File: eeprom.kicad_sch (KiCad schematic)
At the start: 2 parts, among them U8 CAT25320VI-GT3

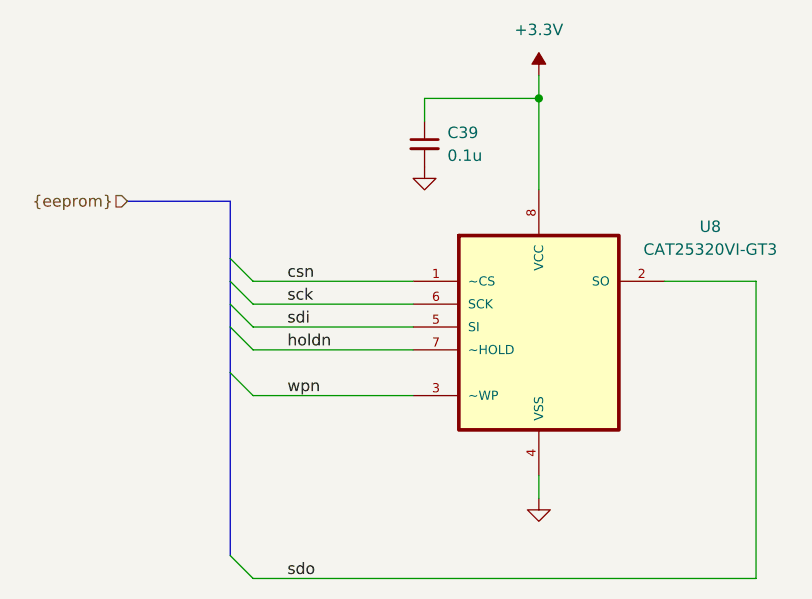
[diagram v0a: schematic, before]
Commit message: Finish BOM
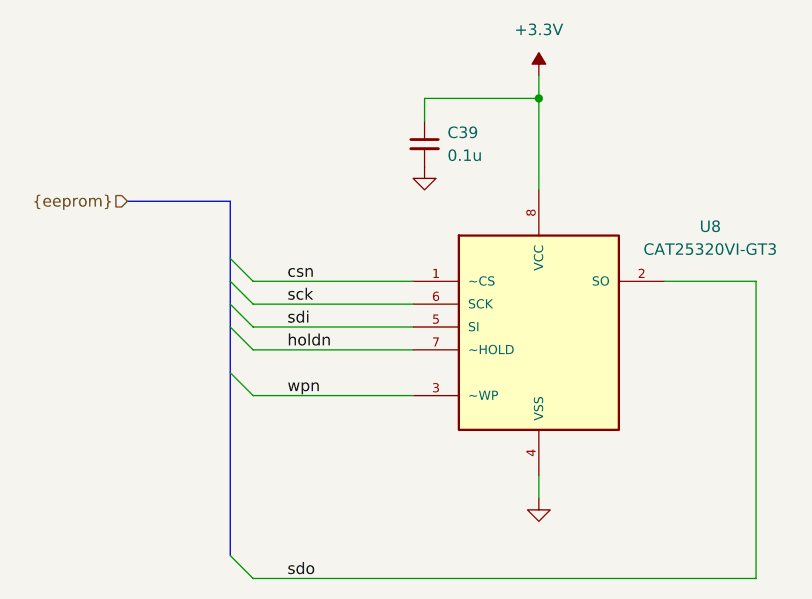
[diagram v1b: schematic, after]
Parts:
- C39: Cost (none) -> .08; MFG (none) -> Taiyo-Yuden; MFG_PN (none) -> TMF212B7104KGHT
- U8: Cost (none) -> 0.55; MFG ON Semiconductor -> ON Semi
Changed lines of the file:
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@@
 			)
 		)
-		(property "Description" "CAT25320VI-GT3 EEPROM Memory, 32kbit, 40ns, 1.8 - 5.5 V 8-Pin SOIC | ON Semiconductor CAT25320VI-GT3"
+		(property "Description" "IC EEPROM 32KBIT SPI 10MHZ 8SOIC"
 			(at 91.948 65.786 0)
 			(effects
@@
 			)
 		)
-		(property "MFG" "ON Semiconductor"
+		(property "MFG" "ON Semi"
 			(at 93.472 61.214 0)
 			(effects
@@
 				)
 				(justify bottom)
+				(hide yes)
+			)
+		)
+		(property "MANUFACTURER_PART_NUMBER" ""
+			(at 91.44 87.63 0)
+			(effects
+				(font
+					(size 1.27 1.27)
+				)
+				(hide yes)
+			)
+		)
+		(property "MFR_NAME" ""
+			(at 91.44 87.63 0)
+			(effects
+				(font
+					(size 1.27 1.27)
+				)
+				(hide yes)
+			)
+		)
+		(property "Part" ""
+			(at 91.44 87.63 0)
+			(effects
+				(font
+					(size 1.27 1.27)
+				)
+				(hide yes)
+			)
+		)
+		(property "Tolerance" ""
+			(at 91.44 87.63 0)
+			(effects
+				(font
+					(size 1.27 1.27)
+				)
+				(hide yes)
+			)
+		)
+		(property "Type" ""
+			(at 91.44 87.63 0)
+			(effects
+				(font
+					(size 1.27 1.27)
+				)
+				(hide yes)
+			)
+		)
+		(property "VENDOR" ""
+			(at 91.44 87.63 0)
+			(effects
+				(font
+					(size 1.27 1.27)
+				)
+				(hide yes)
+			)
+		)
+		(property "Voltage" ""
+			(at 91.44 87.63 0)
+			(effects
+				(font
+					(size 1.27 1.27)
+				)
+				(hide yes)
+			)
+		)
+		(property "Cost" "0.55"
+			(at 91.44 87.63 0)
+			(effects
+				(font
+					(size 1.27 1.27)
+				)
 				(hide yes)
 			)
@@
 			)
 		)
-		(property "Description" "Unpolarized capacitor, small symbol"
-			(at 76.2 64.77 0)
-			(effects
+		(property "Description" "CAP CER 0.1UF 25V X7R 0805"
+			(at 76.2 64.77 0)
+			(effects
+				(font
+					(size 1.27 1.27)
+				)
+				(hide yes)
+			)
+		)
+		(property "MANUFACTURER_PART_NUMBER" ""
+			(at 76.2 64.77 0)
+			(effects
+				(font
+					(size 1.27 1.27)
+				)
+				(hide yes)
+			)
+		)
+		(property "MFR_NAME" ""
+			(at 76.2 64.77 0)
+			(effects
+				(font
+					(size 1.27 1.27)
+				)
+				(hide yes)
+			)
+		)
+		(property "Part" ""
+			(at 76.2 64.77 0)
+			(effects
+				(font
+					(size 1.27 1.27)
+				)
+				(hide yes)
+			)
+		)
+		(property "Tolerance" ""
+			(at 76.2 64.77 0)
+			(effects
+				(font
+					(size 1.27 1.27)
+				)
+				(hide yes)
+			)
+		)
+		(property "Type" ""
+			(at 76.2 64.77 0)
+			(effects
+				(font
+					(size 1.27 1.27)
+				)
+				(hide yes)
+			)
+		)
+		(property "VENDOR" ""
+			(at 76.2 64.77 0)
+			(effects
+				(font
+					(size 1.27 1.27)
+				)
+				(hide yes)
+			)
+		)
+		(property "Voltage" ""
+			(at 76.2 64.77 0)
+			(effects
+				(font
+					(size 1.27 1.27)
+				)
+				(hide yes)
+			)
+		)
+		(property "MFG" "Taiyo-Yuden"
+			(at 76.2 64.77 0)
+			(effects
+				(font
+					(size 1.27 1.27)
+				)
+				(hide yes)
+			)
+		)
+		(property "MFG_PN" "TMF212B7104KGHT"
+			(at 76.2 64.77 0)
+			(effects
+				(font
+					(size 1.27 1.27)
+				)
+				(hide yes)
+			)
+		)
+		(property "Cost" ".08"
+			(at 76.2 64.77 0)
+			(effects
